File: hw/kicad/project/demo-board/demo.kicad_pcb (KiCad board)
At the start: 2 copper layers, 49.5 x 49.5 mm, 21 parts, among them J2 MICRO_SD_HINGE, P1 CONN_01X16, P2 CONN_01X16, SW1 KEY_FLASH, SW2 KEY_RST, U1 NCP1117ST33T3G, U2 ESP-12E

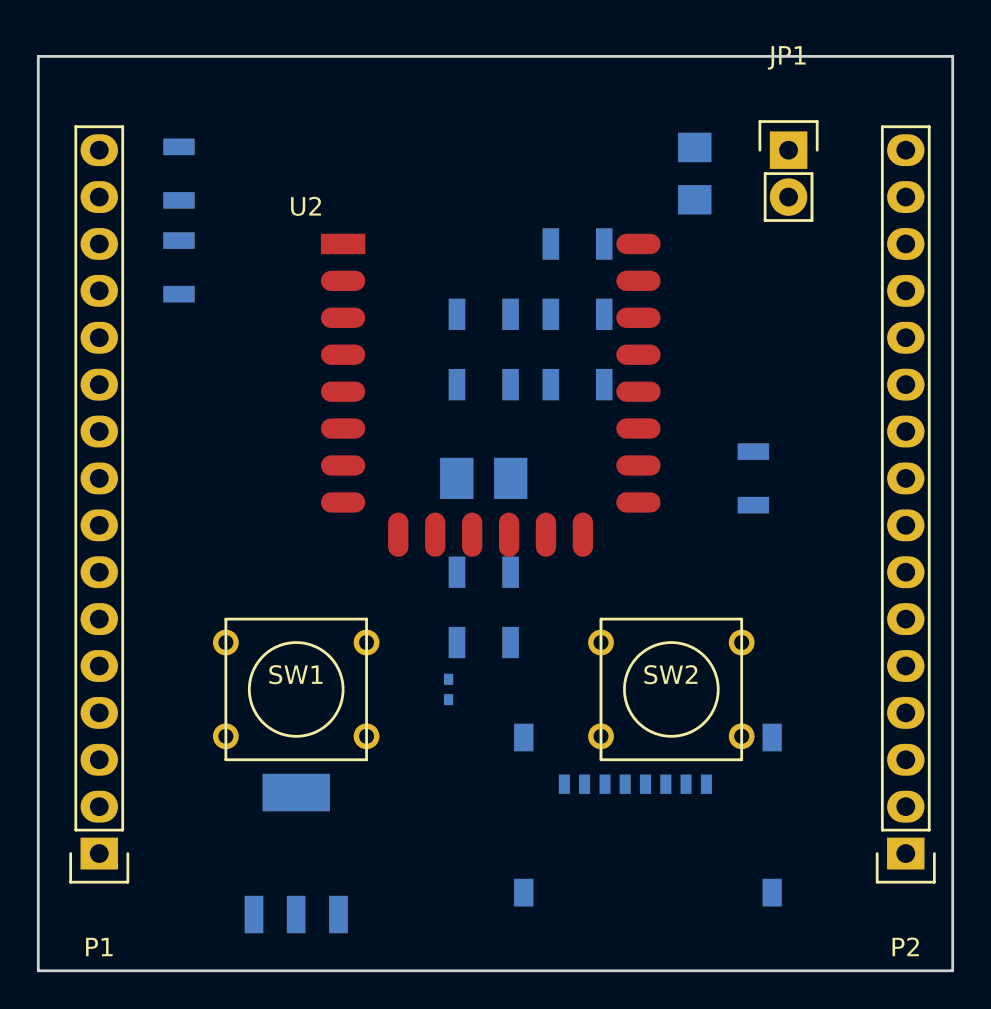
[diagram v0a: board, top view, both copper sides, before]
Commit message: Board routes part 1
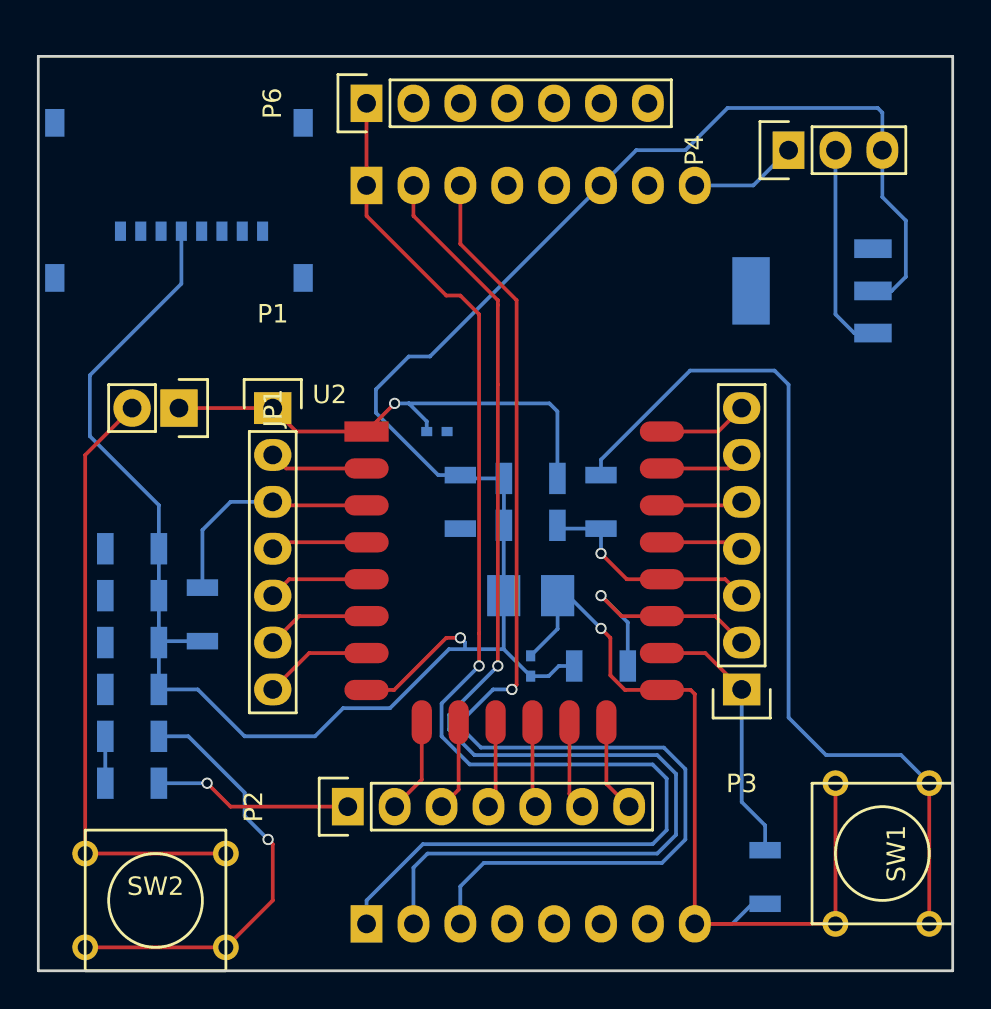
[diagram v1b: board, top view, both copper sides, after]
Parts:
- removed D1: LED, LEDs:LED-1206
- removed R4, R5: 470, Resistors_SMD:R_1206
- added C3: 1nF, Capacitors_SMD:C_0402, B.Cu at (149.9, 102.9)
- added P3: ESP_CONN, Pin_Headers:Pin_Header_Straight_1x07, F.Cu at (161.3, 104.1)
- added P4: PWR_CONN, Pin_Headers:Pin_Header_Straight_1x03, F.Cu at (163.8, 74.9)
- added P5: CONN_DISPLAY, display_local:Nokia_5110_LCD, B.Cu at (141.0, 116.8)
- added P6: SD_LCD_CONN, Pin_Headers:Pin_Header_Straight_1x07, F.Cu at (141.0, 72.4)
- added R11: 50k, Resistors_SMD:R_1206, B.Cu at (146.1, 94.0)
- added R12: 50k, Resistors_SMD:R_1206, B.Cu at (128.3, 99.1)
- added R13: 50k, Resistors_SMD:R_1206, B.Cu at (128.3, 104.1)
- added R14: 50k, Resistors_SMD:R_1206, B.Cu at (128.3, 101.6)
- added R15: 50k, Resistors_SMD:R_1206, B.Cu at (128.3, 96.5)
- P1, P2: value CONN_01X16 -> ESP_CONN; footprint Pin_Headers:Pin_Header_Straight_1x16 -> Pin_Headers:Pin_Header_Straight_1x07
- moved J2 55.1 mm to (130.8, 69.8), turned to 180 degrees
- moved U1 41.3 mm to (165.1, 82.5), turned to 270 degrees
- moved JP1 35.9 mm to (130.8, 88.9), turned to 270 degrees
- moved R2 33.1 mm to (128.3, 109.2), turned to 0 degrees
- moved SW1 33.0 mm to (168.9, 113.0), turned to 270 degrees
- moved P2 30.3 mm to (140.0, 110.5), turned to 90 degrees
- moved SW2 30.2 mm to (129.5, 115.6)
- moved P1 25.9 mm to (135.9, 88.9), turned to 0 degrees
- moved R3 25.5 mm to (128.3, 106.7), turned to 180 degrees
- moved R8 22.3 mm to (132.1, 100.1), turned to 90 degrees
- moved R10 21.6 mm to (162.6, 114.3)
- moved R6 15.5 mm to (149.9, 95.2)
- moved R7 15.3 mm to (153.7, 102.9)
- moved C2 14.0 mm to (144.8, 90.2), turned to 0 degrees
- moved U2 10.2 mm to (141.0, 90.2)
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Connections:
- J2 pad 10: Net-(J2-Pad10) -> GND
- J2 pad 11: Net-(J2-Pad11) -> GND
- J2 pad 12: Net-(J2-Pad12) -> GND
- J2 pad 2: Net-(J2-Pad2) -> /SD_CS
- J2 pad 3: Net-(J2-Pad3) -> /SD_LCD_MOSI
- J2 pad 4: Net-(J2-Pad4) -> VCC
- J2 pad 5: Net-(J2-Pad5) -> /SD_LCD_CLK
- J2 pad 6: Net-(J2-Pad6) -> GND
- J2 pad 7: Net-(J2-Pad7) -> /SD_LCD_MISO
- J2 pad 9: Net-(J2-Pad9) -> GND
- JP1 pad 1: /GPIO16 -> /nRST
- P1 pad 1: /ADC_EX -> /nRST
- P1 pad 3: Net-(P1-Pad3) -> /EN
- P1 pad 4: /GPIO10 -> /GPIO16
- P1 pad 5: /GPIO9 -> /GPIO14
- P1 pad 6: /SPI_INT -> /GPIO12
- P1 pad 7: /SPI_MOSI -> /GPIO13
- P2 pad 1: /GPIO16 -> /ADC_EX
- P2 pad 2: /GPIO5 -> /SPI_MOSI
- P2 pad 3: /GPIO4 -> /SPI_MISO
- P2 pad 4: /GPIO0 -> /GPIO9
- P2 pad 5: /GPIO2 -> /GPIO10
- P2 pad 6: Net-(P2-Pad6) -> /SPI_INT
- P2 pad 7: Net-(P2-Pad7) -> /SPI_CLK
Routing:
- net VCC: track 0.00 -> 128.4 mm, vias 0 -> 1
- net GND: track 0.00 -> 76.1 mm, vias 0 -> 2
- net /LCD_RST: track 0.00 -> 73.1 mm, vias 0 -> 1
- net /LCD_CS: track 0.00 -> 67.1 mm, vias 0 -> 1
- net /SD_LCD_DATA_CMD: track 0.00 -> 64.5 mm, vias 0 -> 1
- net Net-(R1-Pad2): track 0.00 -> 48.1 mm
- net Net-(JP1-Pad2): track 0.00 -> 32.8 mm
- net /nRST: track 0.00 -> 27.4 mm, vias 0 -> 1
- net /GPIO15: track 0.00 -> 14.4 mm
- net /GPIO2: track 0.00 -> 13.1 mm, vias 0 -> 1
- net /EN: track 0.00 -> 12.7 mm
- net /GPIO0: track 0.00 -> 12.3 mm, vias 0 -> 1
- net 5V: track 0.00 -> 11.3 mm
- net /ADC_EX: track 0.00 -> 10.8 mm, vias 0 -> 1
- net /ADC: track 0.00 -> 7.92 mm
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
